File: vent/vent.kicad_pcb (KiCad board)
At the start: 2 copper layers, 31 parts, among them J1 Valve Control, J2 CAN Connector, J3 Programming Header, J4 Valve Connection, Q1 Q_NMOS_GDS, U1 INA180, U2 MCP2562, U3 PIC18F26K83, Y1 Crystal

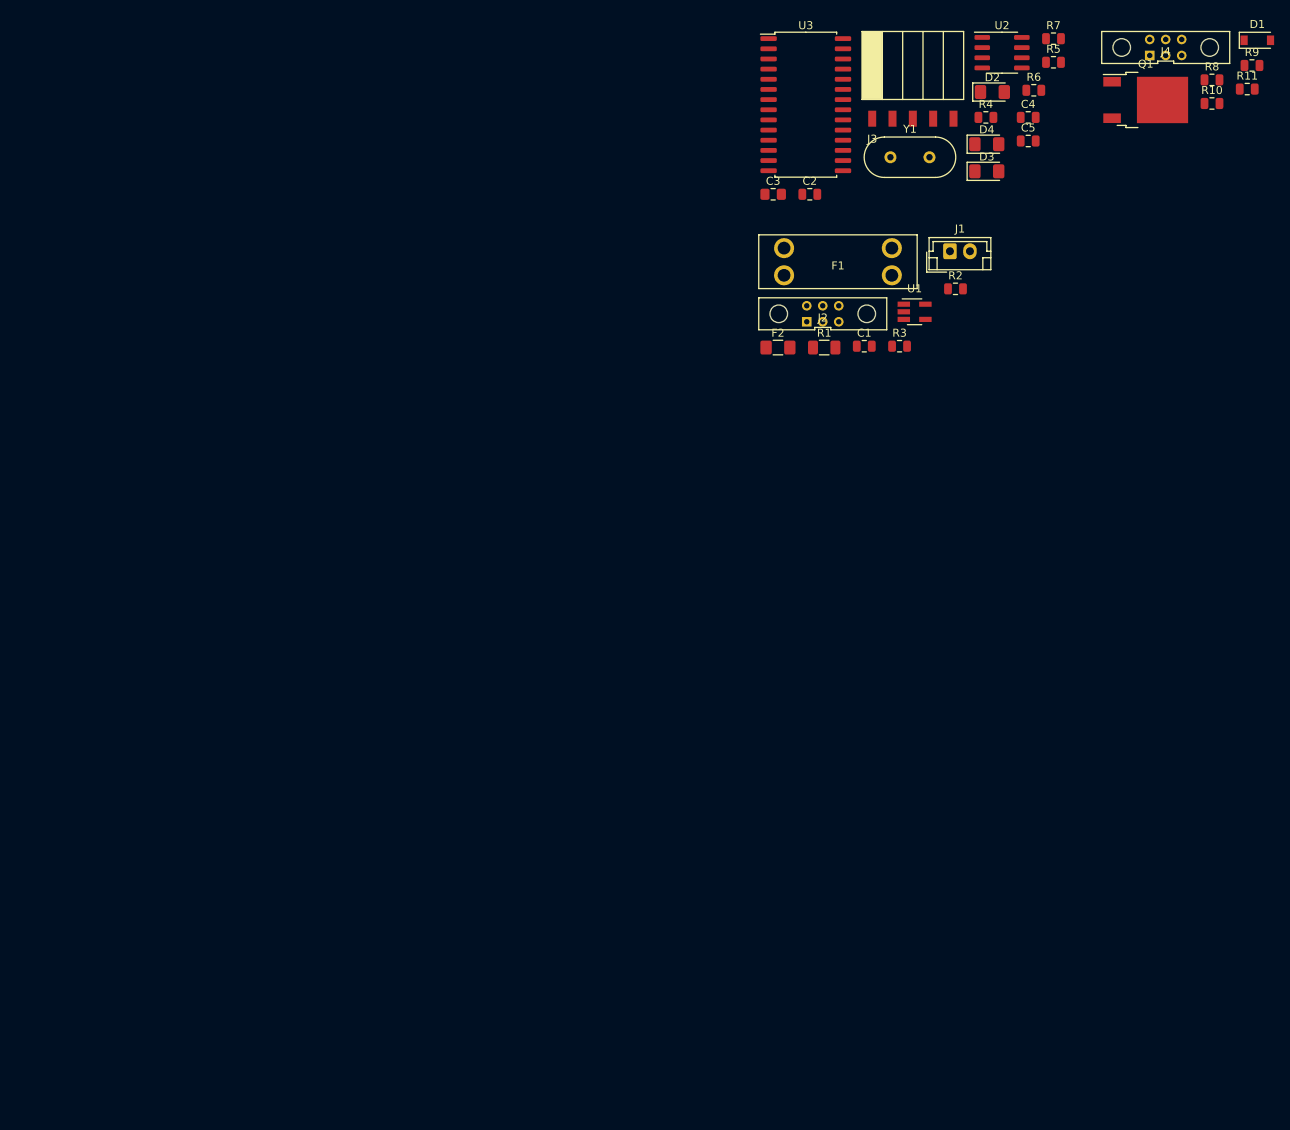
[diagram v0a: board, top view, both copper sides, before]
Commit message: Finish layout
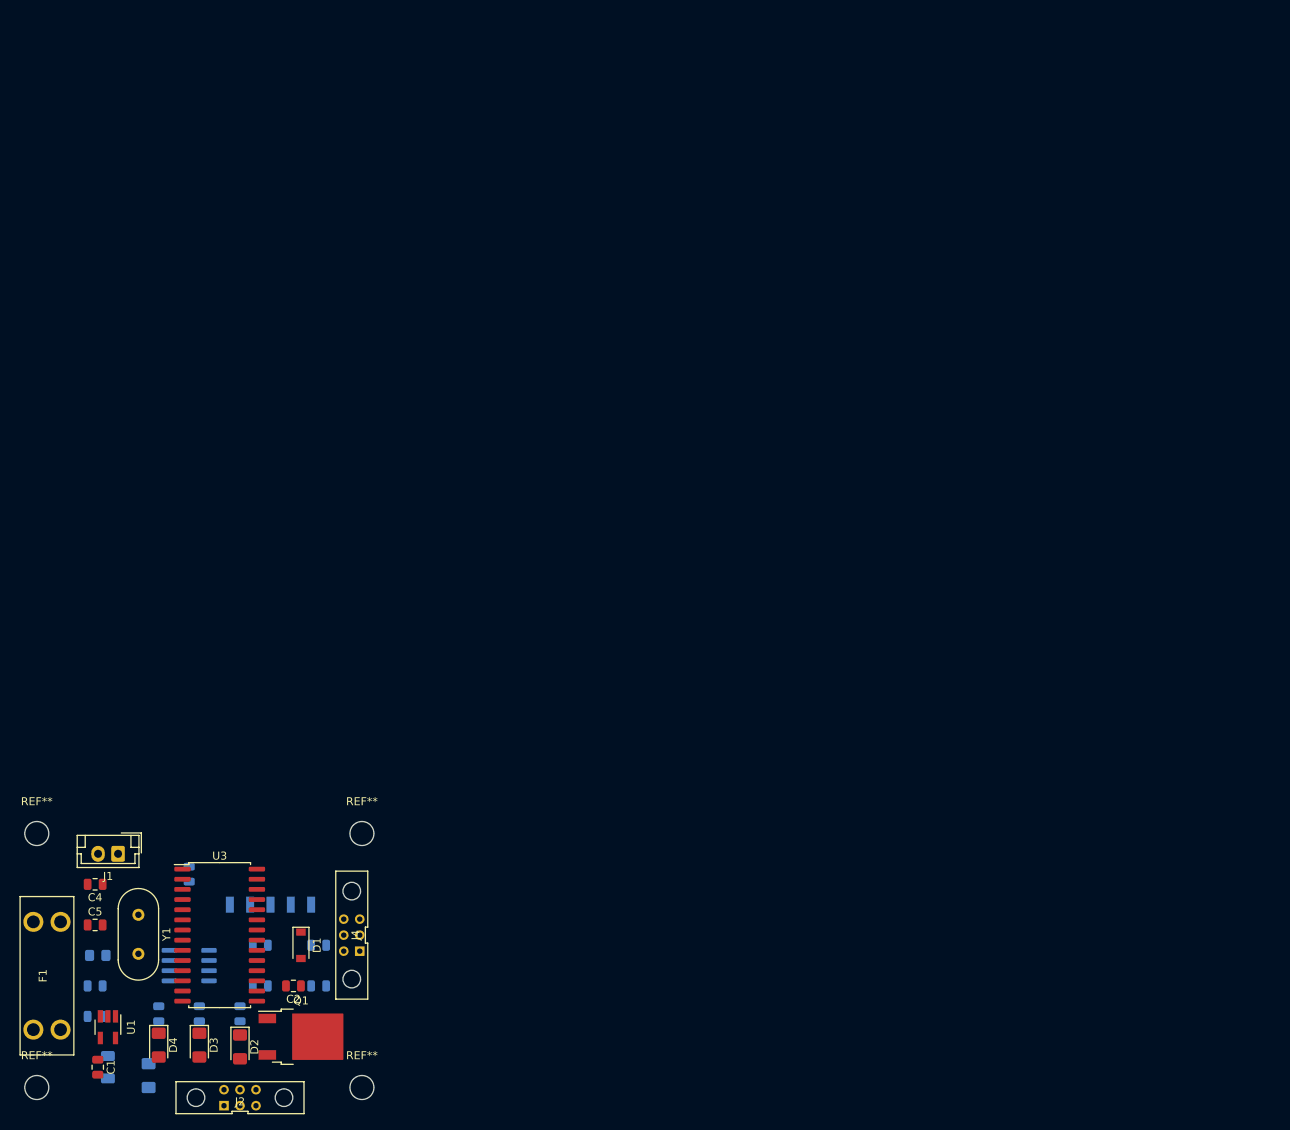
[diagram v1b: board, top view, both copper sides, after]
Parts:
- added REF**: MountingHole_3mm, MountingHole:MountingHole_3mm, F.Cu at (109.2, 133.3)
- added REF**: MountingHole_3mm, MountingHole:MountingHole_3mm, F.Cu at (149.9, 133.3)
- added REF**: MountingHole_3mm, MountingHole:MountingHole_3mm, F.Cu at (109.2, 101.6)
- added REF**: MountingHole_3mm, MountingHole:MountingHole_3mm, F.Cu at (149.9, 101.6)
- C3, F2, J3, R1, R10, R11, R2, R3, R4, R5, R6, R7, R8, R9, U2: moved to B.Cu
- moved R9 165.7 mm to (137.2, 115.6), turned to 180 degrees
- moved R7 165.4 mm to (124.5, 124.1), turned to 270 degrees
- moved D1 164.6 mm to (142.2, 115.6), turned to 270 degrees
- moved R8 164.2 mm to (137.2, 120.7), turned to 180 degrees
- moved R11 157.9 mm to (144.4, 115.6)
- moved Q1 157.7 mm to (142.2, 127.0)
- moved R10 157.0 mm to (144.4, 120.7)
- moved R5 156.5 mm to (134.6, 124.1), turned to 270 degrees
- moved R6 155.6 mm to (129.5, 124.1), turned to 270 degrees
- moved D4 153.0 mm to (124.5, 128.1), turned to 270 degrees
- moved U2 152.8 mm to (128.3, 118.1), turned to 180 degrees
- moved C5 152.3 mm to (116.5, 113.0)
- moved D2 152.0 mm to (134.6, 128.3), turned to 270 degrees
- moved C4 151.0 mm to (116.5, 108.0), turned to 180 degrees
- moved J4 150.5 mm to (148.6, 114.3), turned to 90 degrees
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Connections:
- U3 pad 11: /MCU/CAN_TX -> /MCU/CAN_RX
- U3 pad 12: /MCU/CAN_RX -> /MCU/CAN_TX
